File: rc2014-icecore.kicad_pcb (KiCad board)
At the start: 2 copper layers, 99.3 x 60.1 mm, 21 parts, among them J1 Conn_01x39, J2 Conn_01x10, J3 Conn_02x15_Odd_Even, J4 Conn_02x13_Odd_Even, U1 LM1117-3.3, U2 SN74CB3T3245, U3 SN74CB3T3245, U4 SN74CB3T3245, U5 SN74CB3T3245, U6 SN74CB3T3245

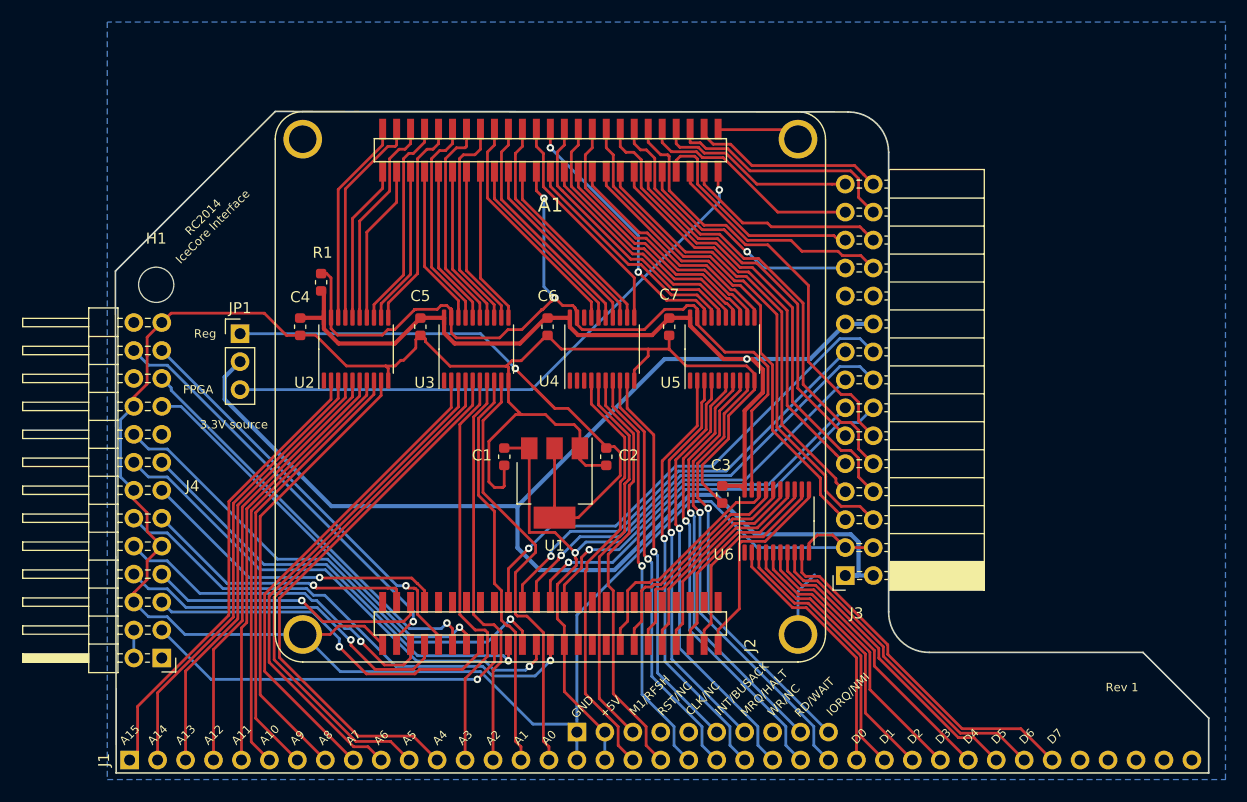
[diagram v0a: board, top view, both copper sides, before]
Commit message: WIP of level shifter
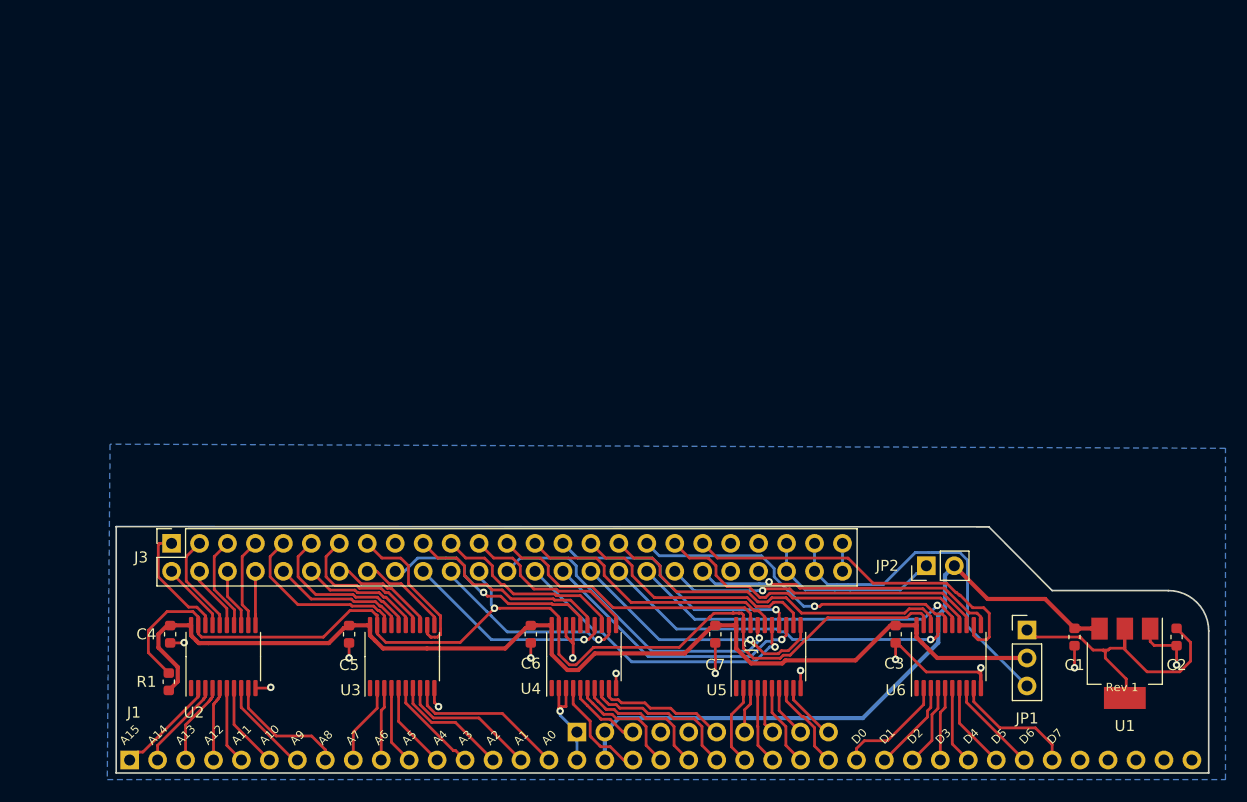
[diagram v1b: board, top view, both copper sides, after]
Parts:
- removed A1: BE-CARRIER, blackedge:BE-CARRIER-SMD
- removed H1: MountingHole, MountingHole:MountingHole_3.2mm_M3
- removed J4: Conn_02x13_Odd_Even, Connector_PinHeader_2.54mm:PinHeader_2x13_P2.54mm_Horizontal
- added JP2: Jumper, Connector_PinHeader_2.54mm:PinHeader_1x02_P2.54mm_Vertical, F.Cu at (134.1, 145.7)
- added REF**: OSHW-Symbol_6.7x6mm_SilkScreen, Symbol:OSHW-Symbol_6.7x6mm_SilkScreen, B.Cu at (152.4, 155.2)
- J3: value Conn_02x15_Odd_Even -> Conn_02x25_Odd_Even; footprint Connector_PinSocket_2.54mm:PinSocket_2x15_P2.54mm_Horizontal -> Connector_PinSocket_2.54mm:PinSocket_2x25_P2.54mm_Vertical
- moved JP1 76.4 mm to (143.3, 151.5)
- moved J3 61.3 mm to (65.5, 143.6), turned to 90 degrees
- moved C1 54.3 mm to (147.6, 152.1)
- moved C2 54.3 mm to (156.8, 152.1)
- moved U1 54.3 mm to (152.1, 154.5)
- moved R1 38.8 mm to (65.3, 156.2)
- moved U2 30.4 mm to (70.2, 153.9)
- moved C4 30.3 mm to (65.4, 151.9)
- moved U3 28.7 mm to (86.5, 153.9)
- moved C5 28.7 mm to (81.7, 151.9)
- moved U5 28.3 mm to (119.8, 153.9)
- moved C7 28.3 mm to (114.9, 151.9)
- moved U4 28.0 mm to (103.0, 153.9)
- moved C6 28.0 mm to (98.2, 151.9)
- moved C3 20.2 mm to (131.3, 151.9)
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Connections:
- J2 pad 8: (no net) -> /~BUSREQ
- J3 pad 1: +3V3 -> /P0
- J3 pad 10: /P36 -> /P9
- J3 pad 11: /P39 -> /P10
- J3 pad 12: /P37 -> /P11
- J3 pad 13: /AN9 -> /P12
- J3 pad 14: /AN8 -> /P13
- J3 pad 15: +5V -> /P14
- J3 pad 16: /AN7 -> /P15
- J3 pad 17: /AN6 -> (no net)
- J3 pad 18: /AN5 -> /P17
- J3 pad 19: +3V3 -> /P18
- J3 pad 2: +3V3 -> /P1
- J3 pad 20: +3V3 -> /P19
- J3 pad 21: GND -> /P20
- J3 pad 22: GND -> /P21
- J3 pad 23: /P42 -> /P22
- J3 pad 24: /P46 -> /P23
- J3 pad 25: /P43 -> /P24
- J3 pad 26: /P47 -> /P25
- J3 pad 27: /P40 -> /P26
- J3 pad 28: /P44 -> /P27
- J3 pad 29: /P41 -> /P28
- J3 pad 3: GND -> /P2
- J3 pad 30: /P45 -> /P29
- J3 pad 4: GND -> /P3
- J3 pad 5: /P34 -> /P4
- J3 pad 6: /P32 -> /P5
- J3 pad 7: /P35 -> /P6
- J3 pad 8: /P33 -> /P7
- J3 pad 9: /P38 -> /P8
- U2 pad 11: /P8 -> /P7
- U2 pad 14: /P3 -> /P4
- U2 pad 15: /P4 -> /P3
- U3 pad 14: /P11 -> /P12
- U3 pad 15: /P12 -> /P11
- U3 pad 18: /P7 -> /P8
- U4 pad 11: /P21 -> /P22
- U4 pad 12: /P22 -> /P21
- U4 pad 15: /P17 -> /P18
- U4 pad 16: /P18 -> /P17
- U4 pad 17: /P16 -> GND
- U4 pad 18: (no net) -> GND
- U4 pad 2: (no net) -> GND
- U4 pad 3: (no net) -> GND
- U5 pad 12: /P29 -> /P30
- U5 pad 13: /P30 -> /P29
- U5 pad 16: /P25 -> /P26
- U5 pad 17: /P26 -> /P25
- U5 pad 5: (no net) -> /~BUSREQ
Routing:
- net GND: track 257.3 -> 51.0 mm, vias 0 -> 14
- net +3V3: track 188.6 -> 100.5 mm, vias 1 -> 0
- net /P32: track 48.4 -> 0.00 mm
- net /TDI: track 46.2 -> 0.00 mm, vias 1 -> 0
- net /TCK: track 45.8 -> 0.00 mm, vias 1 -> 0
- net /TDO: track 45.7 -> 0.00 mm, vias 1 -> 0
- net /AN5: track 45.4 -> 0.00 mm, vias 1 -> 0
- net /P33: track 45.1 -> 0.00 mm
- net /A4: track 50.6 -> 7.99 mm
- net /P34: track 42.5 -> 0.00 mm
- net /P36: track 42.0 -> 0.00 mm
- net /A5: track 48.6 -> 7.20 mm
- net /AN7: track 41.2 -> 0.00 mm, vias 1 -> 0
- net /TMS: track 40.5 -> 0.00 mm, vias 1 -> 0
- net /AN6: track 40.0 -> 0.00 mm, vias 1 -> 0
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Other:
- board size 99.3 x 60.1 mm -> 99.3 x 22.4 mm
- board text added: "SN74CB3T3245 FPGA Level Translator"
- board text removed: "3.3V source"
- board text removed: "FPGA"
- board text removed: "RC2014 IceCore Interface"
- board text removed: "Reg"
- board text removed: "github.com/electrified/rc2014-fpga-interface"
